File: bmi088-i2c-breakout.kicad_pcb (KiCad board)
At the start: 2 copper layers, 14.2 x 9.9 mm, 11 parts, among them J1 Conn_01x04_Socket, J2 Conn_01x04_Socket, U1 BMI088

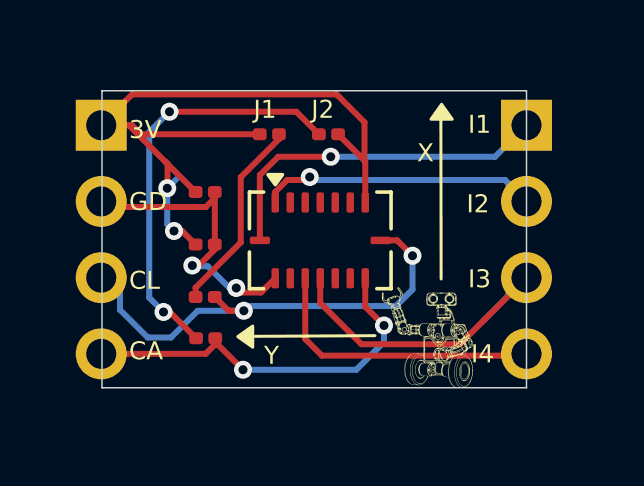
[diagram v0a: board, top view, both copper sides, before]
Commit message: modified:   bmi088-i2c-breakout.kicad_pcb
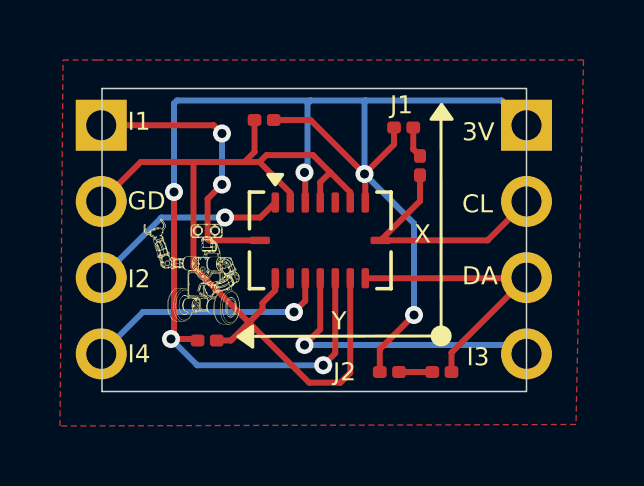
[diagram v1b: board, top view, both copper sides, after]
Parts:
- moved R1 8.39 mm to (155.4, 92.0), turned to -90 degrees
- moved JP1 8.18 mm to (154.4, 98.8), turned to 0 degrees
- moved G*** 8.15 mm to (147.9, 95.5)
- moved R2 7.95 mm to (156.2, 98.8)
- moved JP2 4.48 mm to (154.9, 90.7)
- moved C2 3.20 mm to (148.4, 97.8)
- moved C1 3.10 mm to (150.3, 90.5), turned to 180 degrees
- moved G*** 1.03 mm to (152.5, 94.3)
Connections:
- J1 pad 1: /INT1 -> /3V3
- J1 pad 2: /INT2 -> /SCL
- J1 pad 3: /INT3 -> /SDA
- J1 pad 4: /INT4 -> /INT3
- J2 pad 1: /3V3 -> /INT1
- J2 pad 3: /SCL -> /INT2
- J2 pad 4: /SDA -> /INT4
- U1 pad 11: /VDDIO -> /3V3
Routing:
- net /3V3: track 25.9 -> 50.5 mm, vias 2 -> 6
- net /GND: track 9.87 -> 31.0 mm, vias 2 -> 0
- net Net-(JP1-B): track 13.9 -> 1.11 mm, vias 2 -> 0
- net /SCL: track 15.6 -> 8.12 mm, vias 2 -> 0
- net Net-(JP2-B): track 6.58 -> 1.04 mm
- net /SDA: track 12.3 -> 9.56 mm, vias 2 -> 0
- net /INT2: track 9.02 -> 6.84 mm
- net /INT1: track 11.5 -> 9.62 mm, vias 1 -> 2
- net /INT4: track 9.65 -> 8.28 mm, vias 0 -> 1
- net /INT3: track 11.0 -> 10.0 mm, vias 0 -> 1
- added copper zone on F.Cu, net /GND
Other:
- board size 14.2 x 9.9 mm -> 14.2 x 10.1 mm
- board text added: "DA"
- board text removed: "CA"
